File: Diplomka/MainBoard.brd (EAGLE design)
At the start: 100 x 80 mm, 29 parts, among them K1 ARK550/2, K2 ARK550/2, Q1 AP2012P3C-P22, Q2 BC817-40LT1SMD, SW1 TACTB-64K-F, SW2 TACTB-64K-F, SW3 TACTB-64K-F, U1 ESP32-WROOM-32, U2 AMS1117-3.3

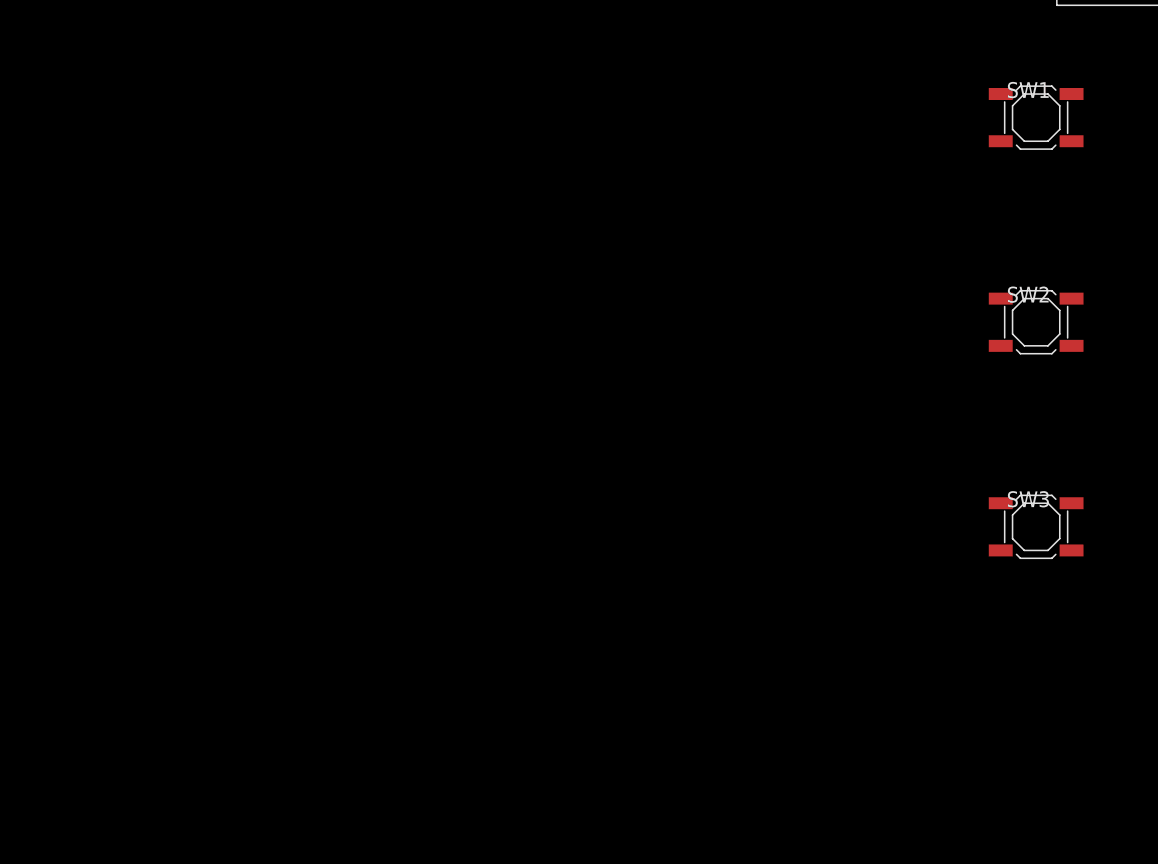
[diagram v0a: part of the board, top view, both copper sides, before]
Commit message: Schema v1.0 hotovo
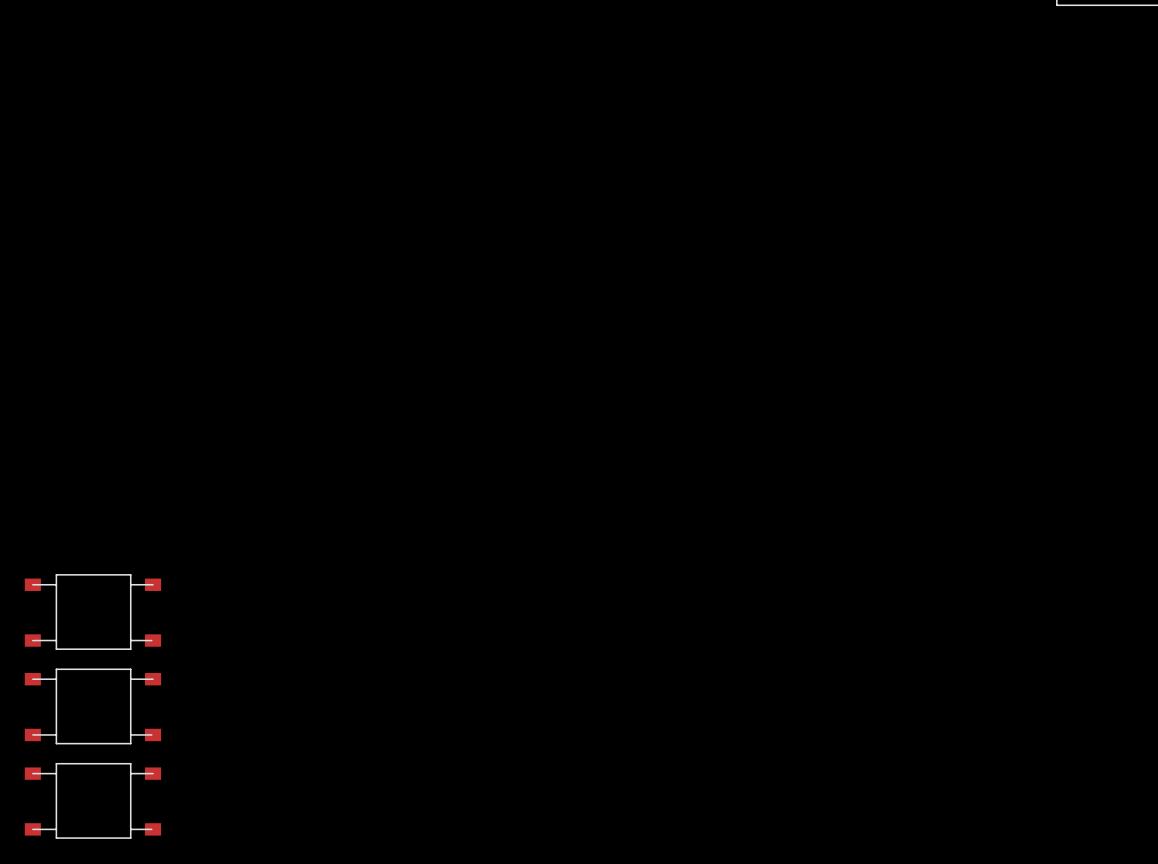
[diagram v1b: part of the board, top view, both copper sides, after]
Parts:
- removed SW1, SW2, SW3: TACTB-64K-F, #PaJa_prepinace:TACTB-64K-F
- added U$6, U$7, U$8: TS6604B, myParts:TS6604B
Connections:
- new net N$9: R10.1
- net BTN_OUTPUT: now also U$8.+; no longer SW3.1
- net GND: now also U$6.-, U$7.-, U$8.-; no longer SW1.1, SW2.3, SW3.3
- net N$7: now also U$6.+; no longer R10.1, SW1.3
- net N$8: now also U$7.+; no longer SW2.1
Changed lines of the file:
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@@
 <attribute name="VALUE" x="-81.915" y="-44.45" size="1.27" layer="27"/>
-</element>
-<element name="SW1" library="#PaJa_prepinace" package="TACTB-64K-F" value="TACTB-64K-F" x="-2.8575" y="-115.285" smashed="yes">
-<attribute name="NAME" x="-5.2428" y="-113.6948" size="1.27" layer="25"/>
-<attribute name="VALUE" x="-5.2433" y="-118.147" size="1.27" layer="27"/>
 </element>
 <element name="R10" library="rcl" library_urn="urn:adsk.eagle:library:334" package="R0805" package3d_urn="urn:adsk.eagle:package:23553/2" value="10k" x="-81.28" y="-57.15" smashed="yes">
@@
 <attribute name="VALUE" x="-81.915" y="-66.04" size="1.27" layer="27"/>
 </element>
-<element name="SW2" library="#PaJa_prepinace" package="TACTB-64K-F" value="TACTB-64K-F" x="-2.8575" y="-131.795" smashed="yes">
-<attribute name="NAME" x="-5.2428" y="-130.2048" size="1.27" layer="25"/>
-<attribute name="VALUE" x="-5.2433" y="-134.657" size="1.27" layer="27"/>
-</element>
 <element name="R12" library="rcl" library_urn="urn:adsk.eagle:library:334" package="R0805" package3d_urn="urn:adsk.eagle:package:23553/2" value="10k" x="-81.28" y="-78.74" smashed="yes">
 <attribute name="NAME" x="-81.915" y="-77.47" size="1.27" layer="25"/>
@@
 <attribute name="VALUE" x="-81.915" y="-81.28" size="1.27" layer="27"/>
 </element>
-<element name="SW3" library="#PaJa_prepinace" package="TACTB-64K-F" value="TACTB-64K-F" x="-2.8575" y="-148.305" smashed="yes">
-<attribute name="NAME" x="-5.2428" y="-146.7148" size="1.27" layer="25"/>
-<attribute name="VALUE" x="-5.2433" y="-151.167" size="1.27" layer="27"/>
-</element>
 <element name="U$5" library="myParts" package="HTU21D" value="HTU21D" x="-83.82" y="-100.33" smashed="yes"/>
+<element name="U$6" library="myParts" package="TS6604B" value="TS6604B" x="-83.82" y="-157.48" smashed="yes"/>
+<element name="U$7" library="myParts" package="TS6604B" value="TS6604B" x="-83.82" y="-165.1" smashed="yes"/>
+<element name="U$8" library="myParts" package="TS6604B" value="TS6604B" x="-83.82" y="-172.72" smashed="yes"/>
 </elements>
 <signals>
@@
 <contactref element="LED1" pad="C"/>
 <contactref element="K1" pad="1"/>
-<contactref element="SW1" pad="1"/>
-<contactref element="SW2" pad="3"/>
-<contactref element="SW3" pad="3"/>
 <contactref element="U$5" pad="GND"/>
 <contactref element="R5" pad="1"/>
@@
 <contactref element="R7" pad="1"/>
 <contactref element="U$1" pad="GND"/>
+<contactref element="U$6" pad="-"/>
+<contactref element="U$7" pad="-"/>
+<contactref element="U$8" pad="-"/>
+<wire x1="-83.82" y1="-157.48" x2="-83.82" y2="-165.1" width="0" layer="19" extent="1-1"/>
+<wire x1="-83.82" y1="-172.72" x2="-83.82" y2="-165.1" width="0" layer="19" extent="1-1"/>
+<wire x1="-82.55" y1="-93.98" x2="-83.82" y2="-157.48" width="0" layer="19" extent="1-1"/>
 <wire x1="-81.28" y1="-34.51" x2="-82.55" y2="-93.98" width="0" layer="19" extent="1-1"/>
 <wire x1="-72.71" y1="-30.31" x2="-81.28" y2="-34.51" width="0" layer="19" extent="1-1"/>
@@
 <wire x1="-58.1" y1="62.23" x2="-44.13" y2="72.39" width="0" layer="19" extent="1-1"/>
 <wire x1="-59.225" y1="41.66" x2="-58.1" y2="62.23" width="0" layer="19" extent="1-1"/>
-<wire x1="-5.715" y1="-113.38" x2="-82.55" y2="-93.98" width="0" layer="19" extent="1-1"/>
-<wire x1="0" y1="-95.22" x2="-5.715" y2="-113.38" width="0" layer="19" extent="1-1"/>
-<wire x1="-5.715" y1="-133.7" x2="-5.715" y2="-113.38" width="0" layer="19" extent="1-1"/>
-<wire x1="-5.715" y1="-150.21" x2="-5.715" y2="-133.7" width="0" layer="19" extent="1-1"/>
+<wire x1="0" y1="-95.22" x2="-82.55" y2="-93.98" width="0" layer="19" extent="1-1"/>
 </signal>
 <signal name="5V">
@@
 </signal>
 <signal name="N$7">
-<contactref element="SW1" pad="3"/>
-<contactref element="R10" pad="1"/>
 <contactref element="U1" pad="3"/>
-<wire x1="-31.36" y1="19.23" x2="-82.23" y2="-57.15" width="0" layer="19" extent="1-1"/>
-<wire x1="-5.715" y1="-117.19" x2="-82.23" y2="-57.15" width="0" layer="19" extent="1-1"/>
+<contactref element="U$6" pad="+"/>
+<wire x1="-31.36" y1="19.23" x2="-83.82" y2="-152.98" width="0" layer="19" extent="1-1"/>
 </signal>
 <signal name="N$8">
 <contactref element="R11" pad="1"/>
 <contactref element="U1" pad="25"/>
-<contactref element="SW2" pad="1"/>
+<contactref element="U$7" pad="+"/>
+<wire x1="-82.23" y1="-63.5" x2="-83.82" y2="-160.6" width="0" layer="19" extent="1-1"/>
 <wire x1="-14.36" y1="5.26" x2="-82.23" y2="-63.5" width="0" layer="19" extent="1-1"/>
-<wire x1="-5.715" y1="-129.89" x2="-82.23" y2="-63.5" width="0" layer="19" extent="1-1"/>
 </signal>
 <signal name="BTN_OUTPUT">
-<contactref element="SW3" pad="1"/>
 <contactref element="R12" pad="1"/>
 <contactref element="U1" pad="13"/>
+<contactref element="U$8" pad="+"/>
+<wire x1="-82.23" y1="-78.74" x2="-83.82" y2="-168.22" width="0" layer="19" extent="1-1"/>
 <wire x1="-31.36" y1="6.53" x2="-82.23" y2="-78.74" width="0" layer="19" extent="1-1"/>
-<wire x1="-5.715" y1="-146.4" x2="-82.23" y2="-78.74" width="0" layer="19" extent="1-1"/>
+</signal>
+<signal name="N$9">
+<contactref element="R10" pad="1"/>
 </signal>
 </signals>
